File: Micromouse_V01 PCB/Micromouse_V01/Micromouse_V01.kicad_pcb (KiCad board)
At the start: 2 copper layers, 70.7 x 100 mm, 73 parts, among them J1 Conn_01x02_Female, J2 Conn_01x02_Female, J3 OLED, J4 Conn_01x02_Female, J5 AS5600 Left, J6 AS5600 Right, J7 Conn_01x02_Female, J8 Conn_01x02_Female, Q1 Q_NPN_BEC, Q2 Q_NPN_BEC, Q3 Q_NPN_BEC, Q4 Q_NPN_BEC, Q5 Q_NPN_BEC, Q6 Q_NPN_BEC, SW1 SW_DPDT_x2, SW2 Start, SW3 Start, U1 AMS1117-3.3, U11 ESP32-WROOM, U12 TB6612FNG, U13 MPU-6050

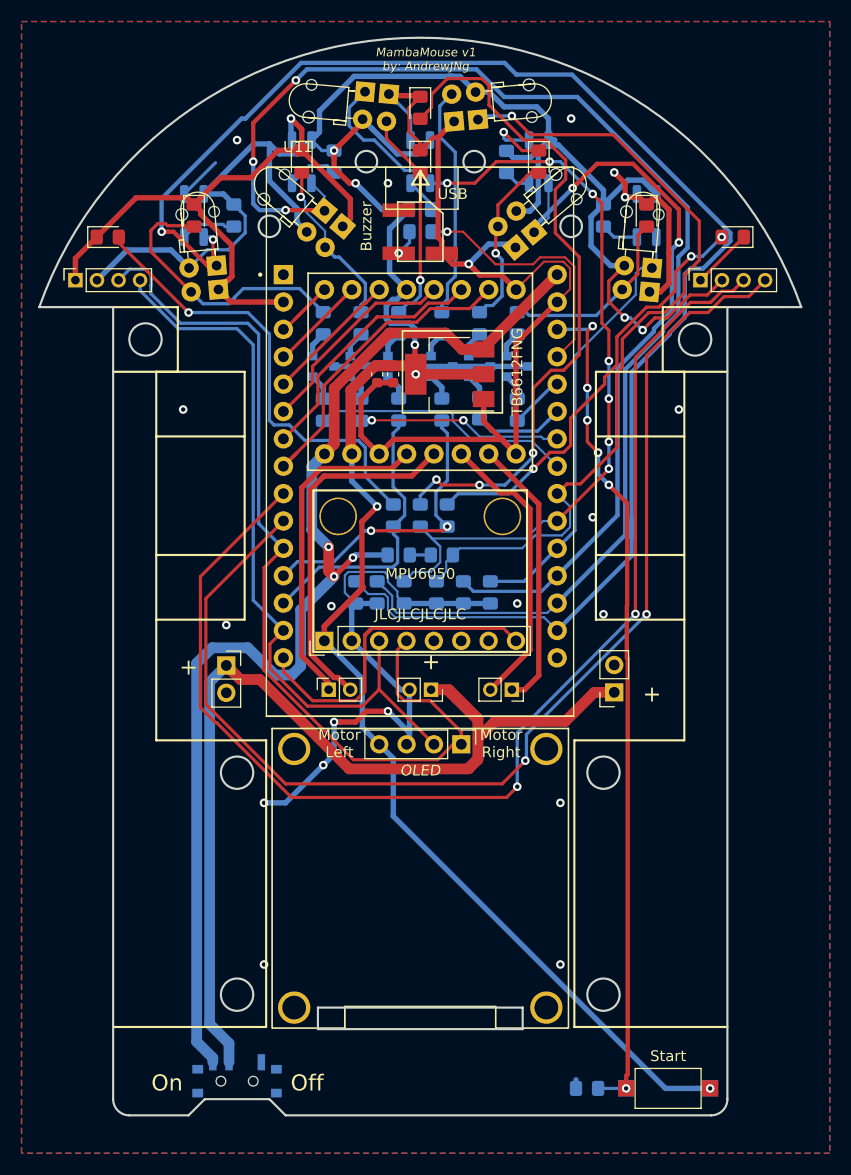
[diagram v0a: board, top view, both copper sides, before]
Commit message: backup after long time, to update kicad
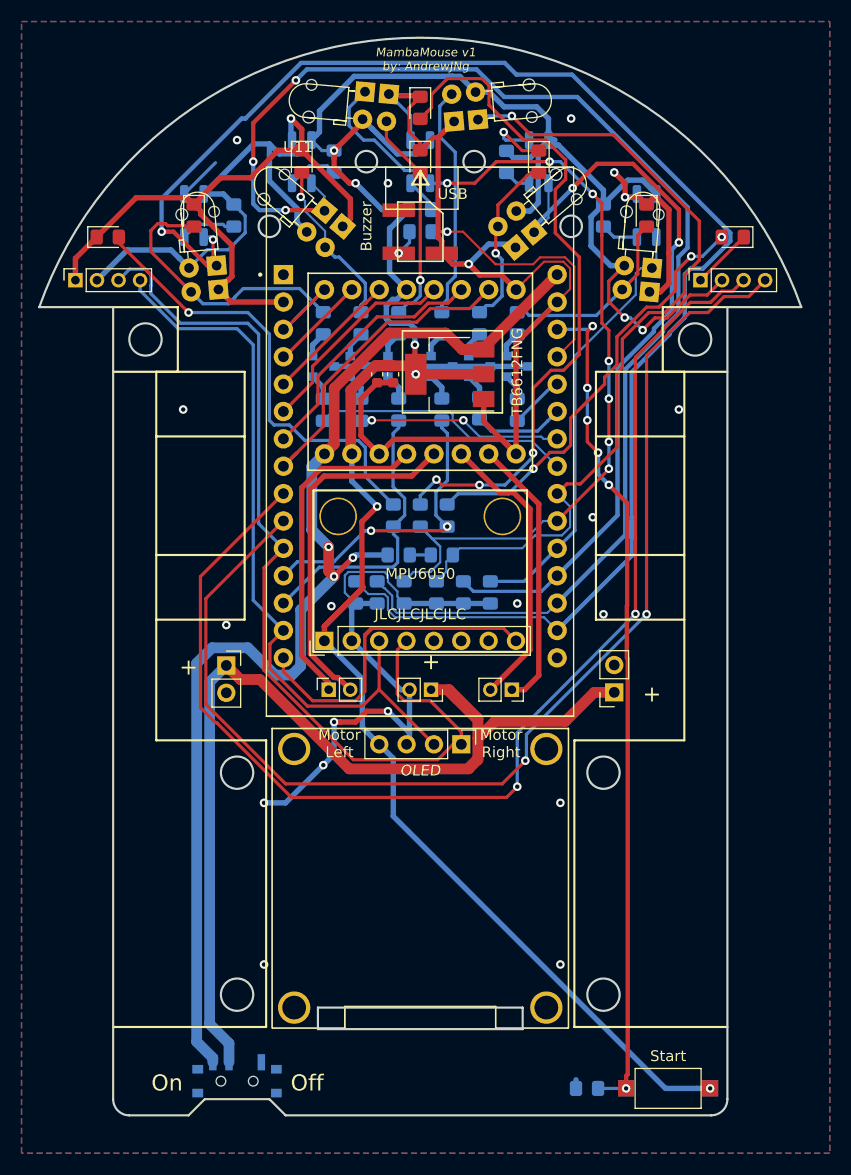
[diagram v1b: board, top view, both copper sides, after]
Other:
- net class Default removed
